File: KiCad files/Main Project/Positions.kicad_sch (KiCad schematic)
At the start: 52 parts

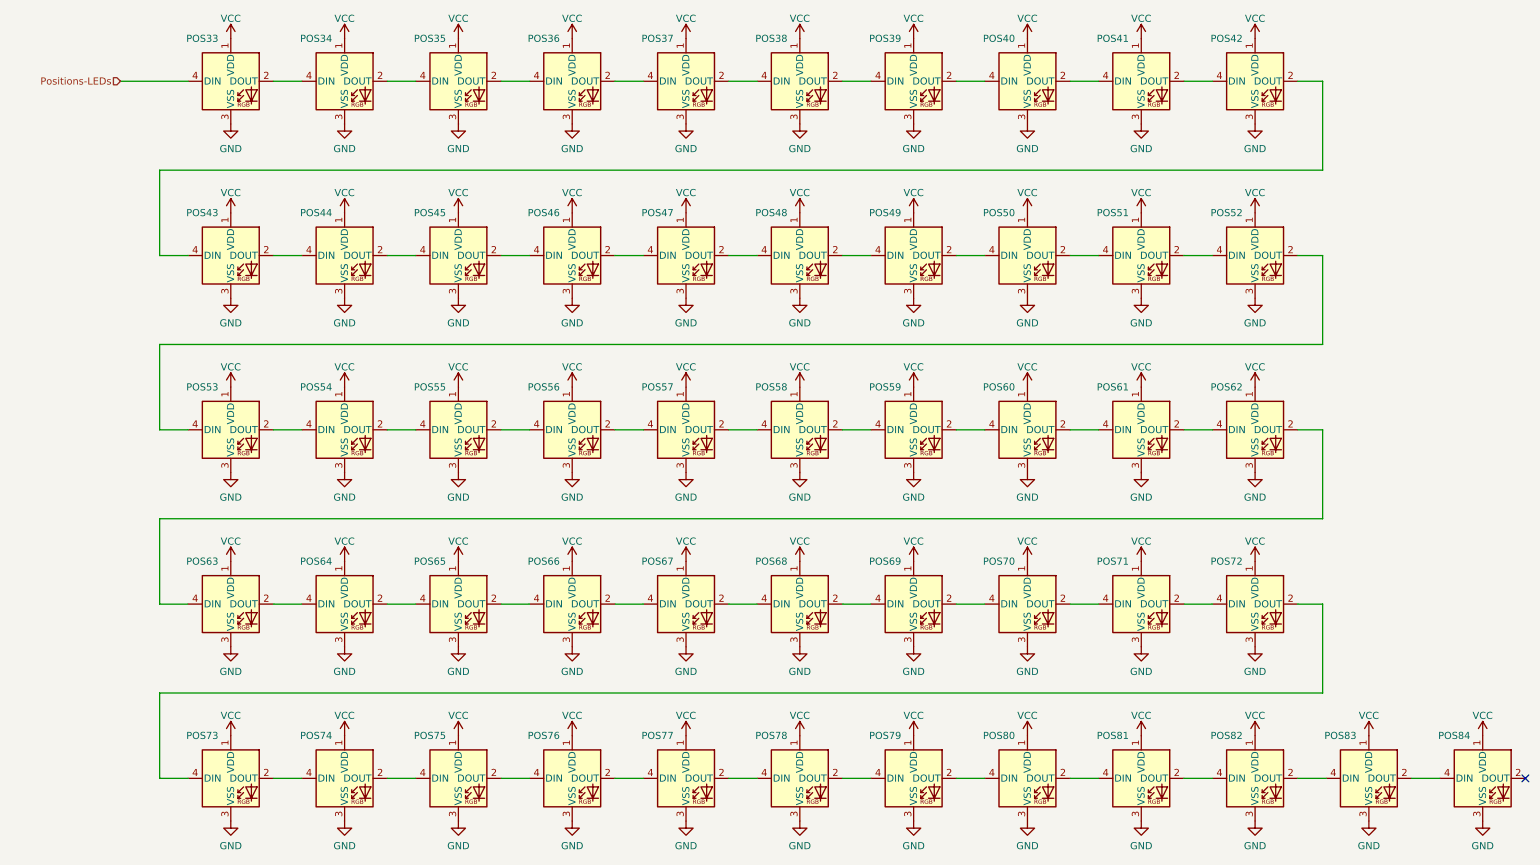
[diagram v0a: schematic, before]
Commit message: update
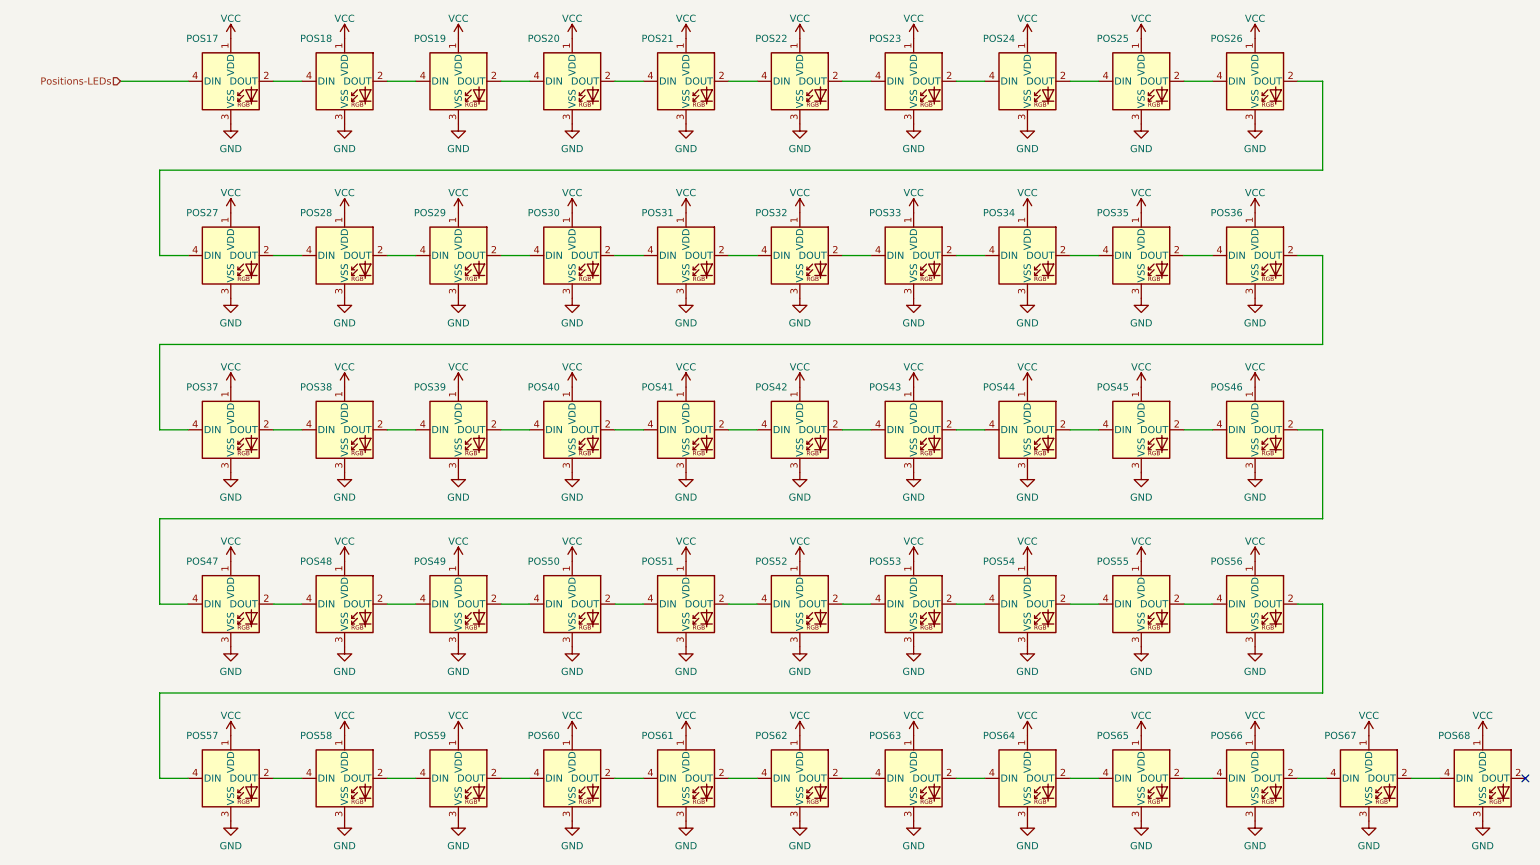
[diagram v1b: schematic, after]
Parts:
- renumbered POS33 to POS17, POS34 to POS18, POS35 to POS19, POS36 to POS20, POS37 to POS21, POS38 to POS22, POS39 to POS23, POS40 to POS24, POS41 to POS25, POS42 to POS26, POS43 to POS27, POS44 to POS28, POS45 to POS29, POS46 to POS30, POS47 to POS31, POS48 to POS32, POS49 to POS33, POS50 to POS34, POS51 to POS35, POS52 to POS36, POS53 to POS37, POS54 to POS38, POS55 to POS39, POS56 to POS40, POS57 to POS41, POS58 to POS42, POS59 to POS43, POS60 to POS44, POS61 to POS45, POS62 to POS46, POS63 to POS47, POS64 to POS48, POS65 to POS49, POS66 to POS50, POS67 to POS51, POS68 to POS52, POS69 to POS53, POS70 to POS54, POS71 to POS55, POS72 to POS56, POS73 to POS57, POS74 to POS58, POS75 to POS59, POS76 to POS60, POS77 to POS61, POS78 to POS62, POS79 to POS63, POS80 to POS64, POS81 to POS65, POS82 to POS66, POS83 to POS67, POS84 to POS68

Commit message: update
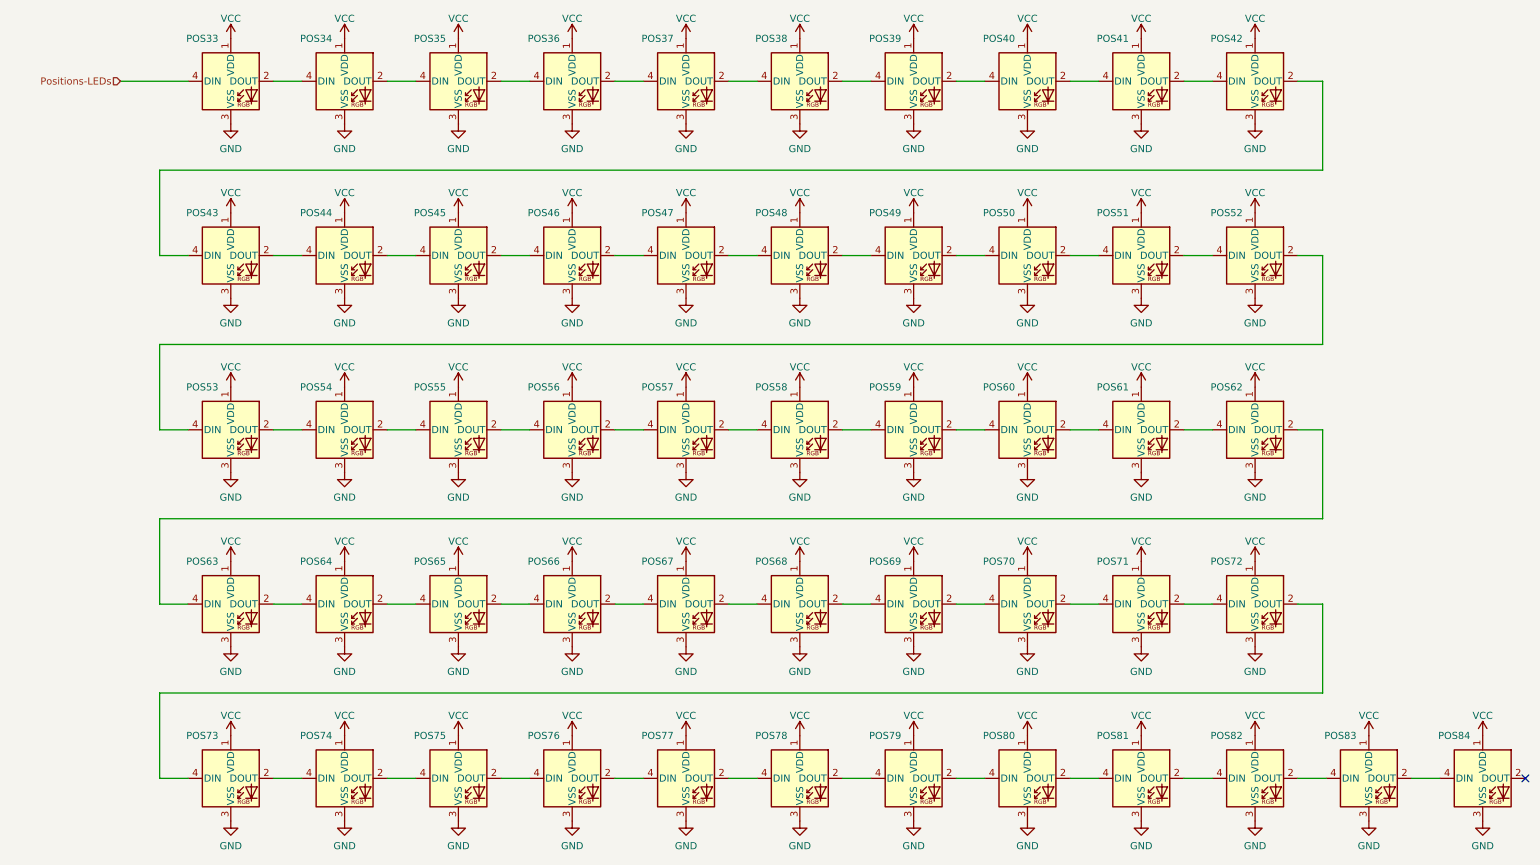
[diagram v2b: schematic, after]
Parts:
- renumbered POS17 to POS33, POS18 to POS34, POS19 to POS35, POS20 to POS36, POS21 to POS37, POS22 to POS38, POS23 to POS39, POS24 to POS40, POS25 to POS41, POS26 to POS42, POS27 to POS43, POS28 to POS44, POS29 to POS45, POS30 to POS46, POS31 to POS47, POS32 to POS48, POS33 to POS49, POS34 to POS50, POS35 to POS51, POS36 to POS52, POS37 to POS53, POS38 to POS54, POS39 to POS55, POS40 to POS56, POS41 to POS57, POS42 to POS58, POS43 to POS59, POS44 to POS60, POS45 to POS61, POS46 to POS62, POS47 to POS63, POS48 to POS64, POS49 to POS65, POS50 to POS66, POS51 to POS67, POS52 to POS68, POS53 to POS69, POS54 to POS70, POS55 to POS71, POS56 to POS72, POS57 to POS73, POS58 to POS74, POS59 to POS75, POS60 to POS76, POS61 to POS77, POS62 to POS78, POS63 to POS79, POS64 to POS80, POS65 to POS81, POS66 to POS82, POS67 to POS83, POS68 to POS84
